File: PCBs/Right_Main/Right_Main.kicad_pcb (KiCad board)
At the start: 2 copper layers, 221 x 111.8 mm, 40 parts, among them J10 Screw_Terminal_01x08, J11 Screw_Terminal_01x08, J12 Screw_Terminal_01x08, J13 Screw_Terminal_01x08, J14 Screw_Terminal_01x08, J15 Screw_Terminal_01x08, J16 Conn_RJ45_Right_To_Left, J2 Screw terminal 5V GND Out, J3 Encoder inputs B, J4 Encoder inputs A, J5 Analog inputs, J7 Conn_Right_Keypad, J8 Rotary switchs' pin 1, U1 MCP23017_SP, U10 MAX485E, U2 ULN2003A, U4 74HC165, U5 74HC165, U6 74HC165, U7 74HC165, U8 74HC165, U9 74HC165

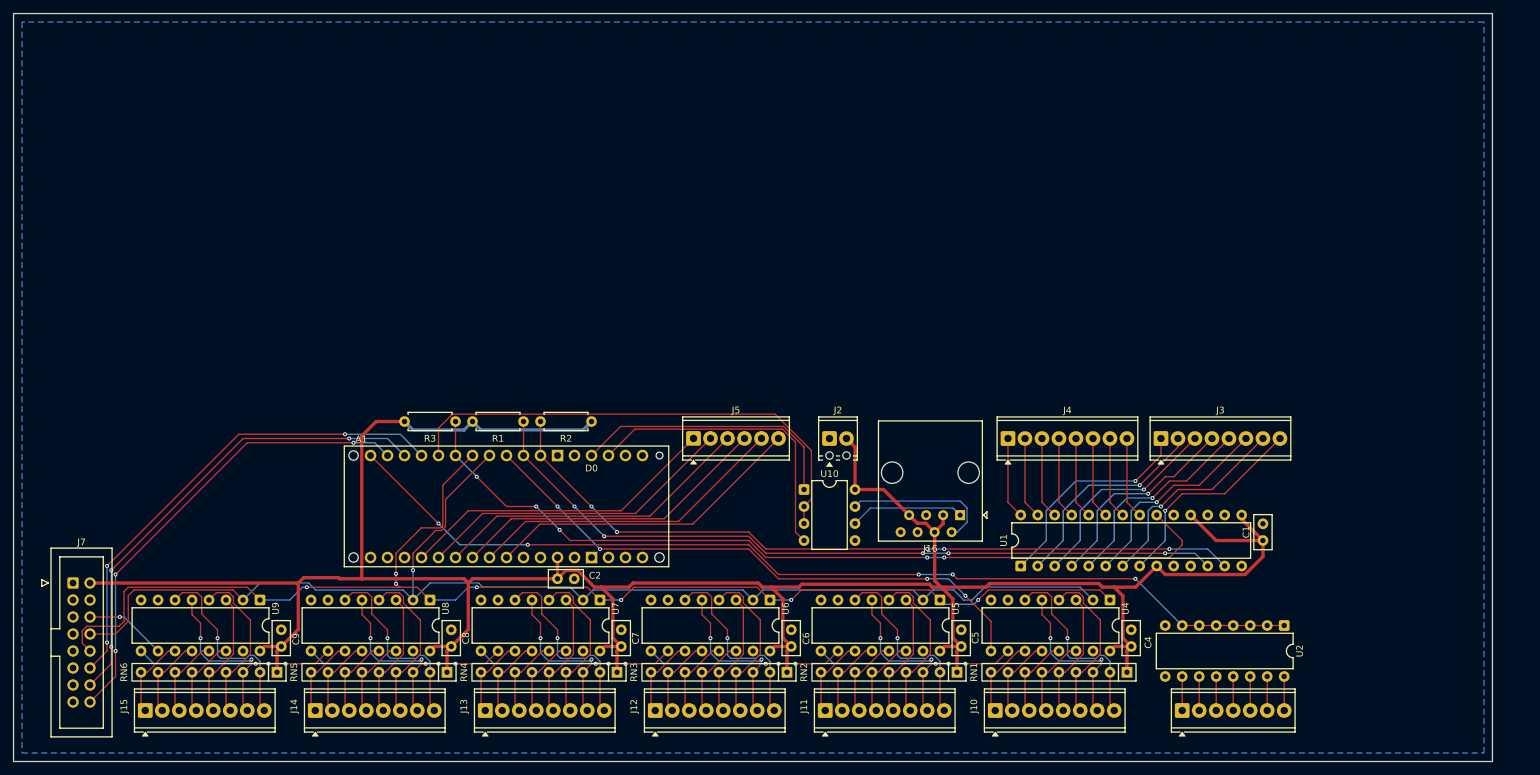
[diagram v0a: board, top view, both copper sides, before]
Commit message: right main pcb draft 2 wip
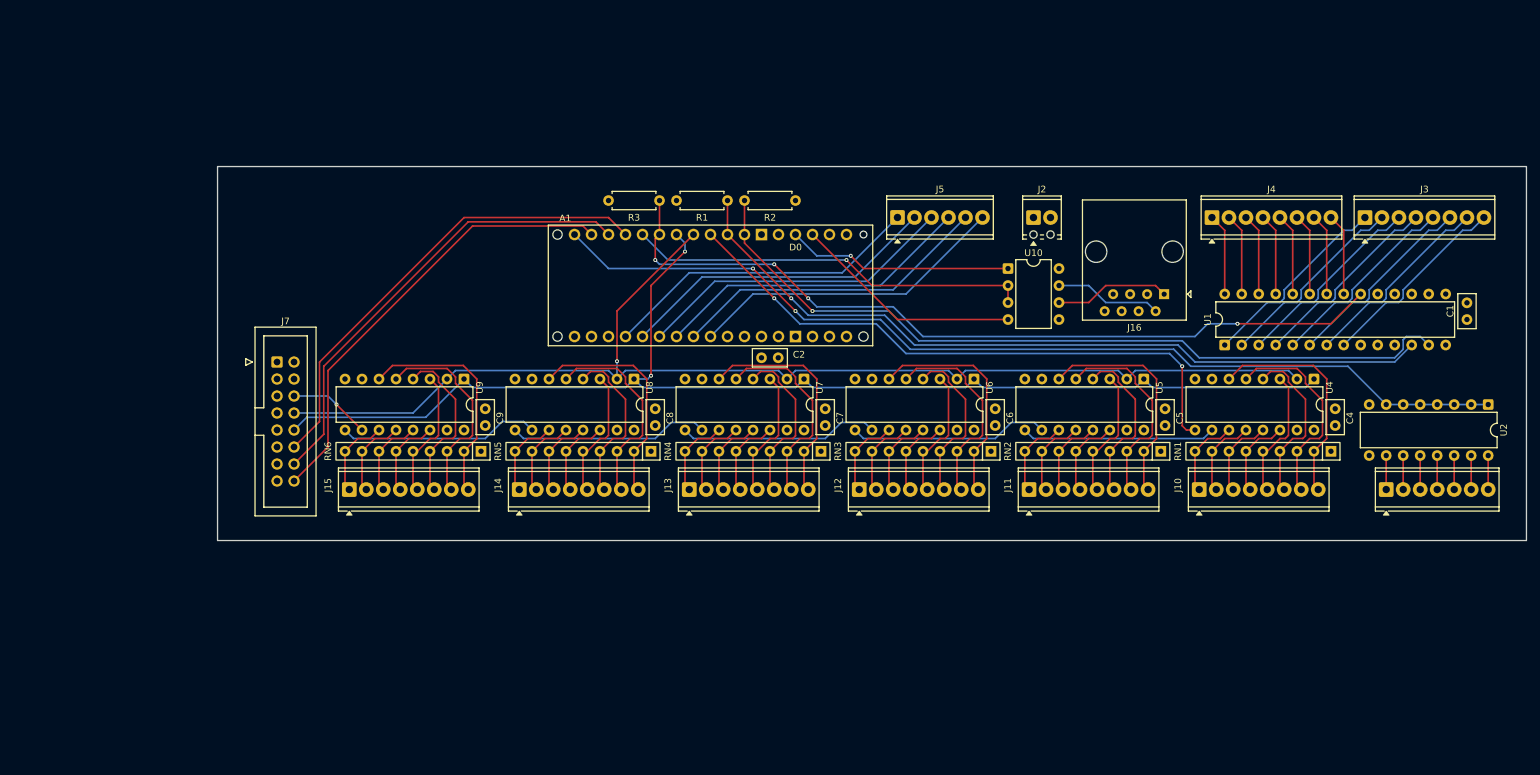
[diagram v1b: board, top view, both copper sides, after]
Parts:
- moved C6 44.9 mm to (179.7, 99.7)
- moved U10 44.9 mm to (181.6, 78.7)
- moved U2 44.9 mm to (253.4, 99.1)
- moved U4 44.9 mm to (227.3, 95.2)
- moved C7 44.9 mm to (154.3, 99.7)
- moved C8 44.9 mm to (128.9, 99.7)
- moved J13 44.9 mm to (134.0, 111.8)
- moved J7 44.9 mm to (72.4, 92.7)
- moved RN1 44.9 mm to (229.9, 106.0)
- moved U1 44.9 mm to (214.0, 90.2)
- moved U8 44.9 mm to (125.7, 95.2)
- moved U9 44.9 mm to (100.3, 95.2)
- moved C4 44.9 mm to (230.5, 99.7)
- moved C9 44.9 mm to (103.5, 99.7)
- moved J16 44.9 mm to (204.9, 82.6)
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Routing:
- net +5V: track 405.0 -> 0.00 mm
- net Net-(U10-DE): track 74.3 -> 60.3 mm, vias 0 -> 1
- net Net-(A1-D1/TX): track 45.6 -> 34.5 mm
- net /Input register 1//PL: track 196.4 -> 187.3 mm, vias 7 -> 2
- net /Input register 1/CP: track 191.8 -> 183.5 mm
- net Net-(A1-D0/RX): track 41.2 -> 33.9 mm, vias 0 -> 1
- net Net-(J16-485_B): track 22.6 -> 16.0 mm
- net Net-(A1-D7_INT4): track 126.8 -> 121.9 mm, vias 5 -> 4
- net Net-(J15-Pin_7): track 25.1 -> 29.7 mm, vias 2 -> 0
- net Net-(J13-Pin_7): track 25.1 -> 29.7 mm, vias 2 -> 0
- net Net-(J14-Pin_7): track 25.1 -> 29.7 mm, vias 2 -> 0
- net Net-(J11-Pin_7): track 25.1 -> 29.7 mm, vias 2 -> 0
- net Net-(J10-Pin_7): track 25.1 -> 29.7 mm, vias 2 -> 0
- net Net-(J12-Pin_7): track 25.1 -> 29.7 mm, vias 2 -> 0
- net Net-(A1-D2/SDA): track 114.2 -> 118.4 mm, vias 5 -> 1
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- added copper zone on In2.Cu, net +5V
- added copper zone on In1.Cu, net GND
- removed copper zone on B.Cu, net GND
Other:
- board size 221 x 111.8 mm -> 195.6 x 55.9 mm
- copper layers 2 -> 4
